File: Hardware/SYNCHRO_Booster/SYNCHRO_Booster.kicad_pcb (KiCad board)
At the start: 2 copper layers, 41 parts, among them IC1 L6203, J1 Conn_01x02_Pin, J2 Power_Input, J3 B4B-XH-A, SW1 SW_Push, SW2 SW_SPDT, U1 LM393P, U2 6N137, U3 6N137, U4 74LVC2G02

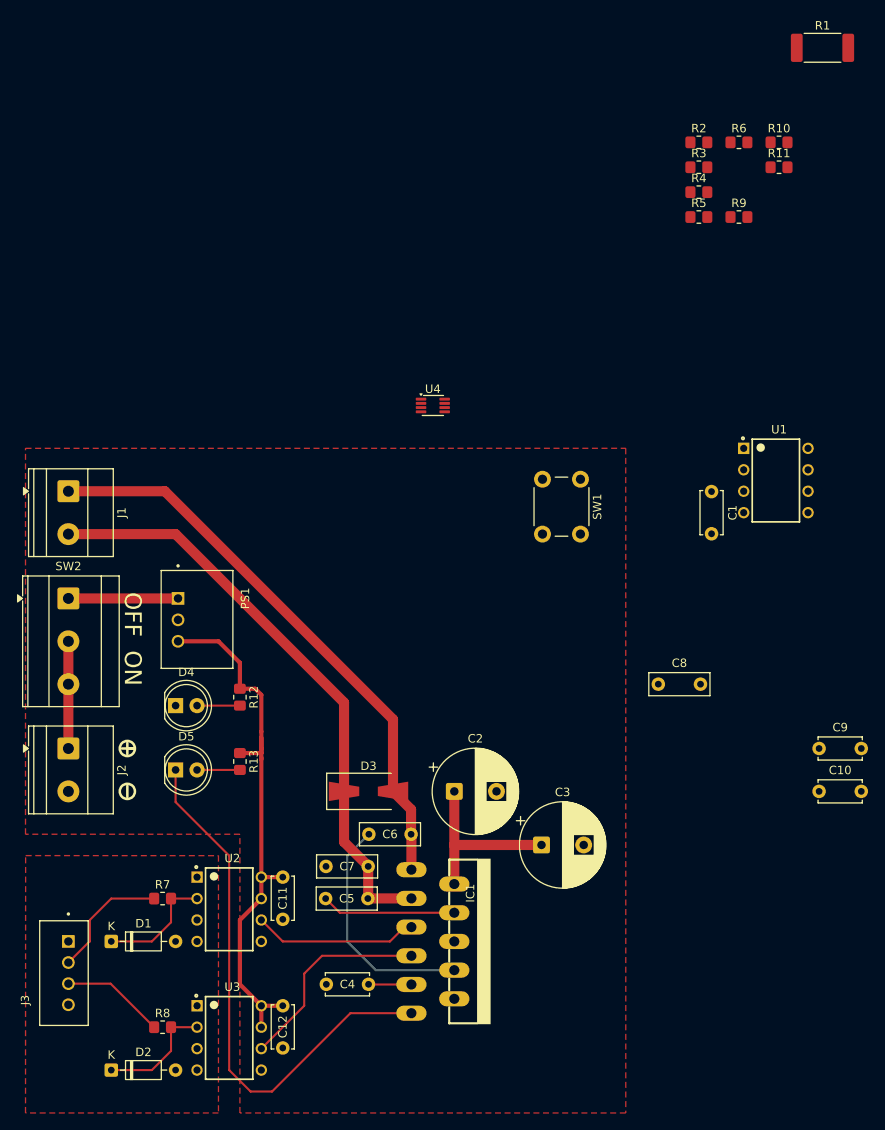
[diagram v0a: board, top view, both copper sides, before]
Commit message: Booster_Design_v1.0
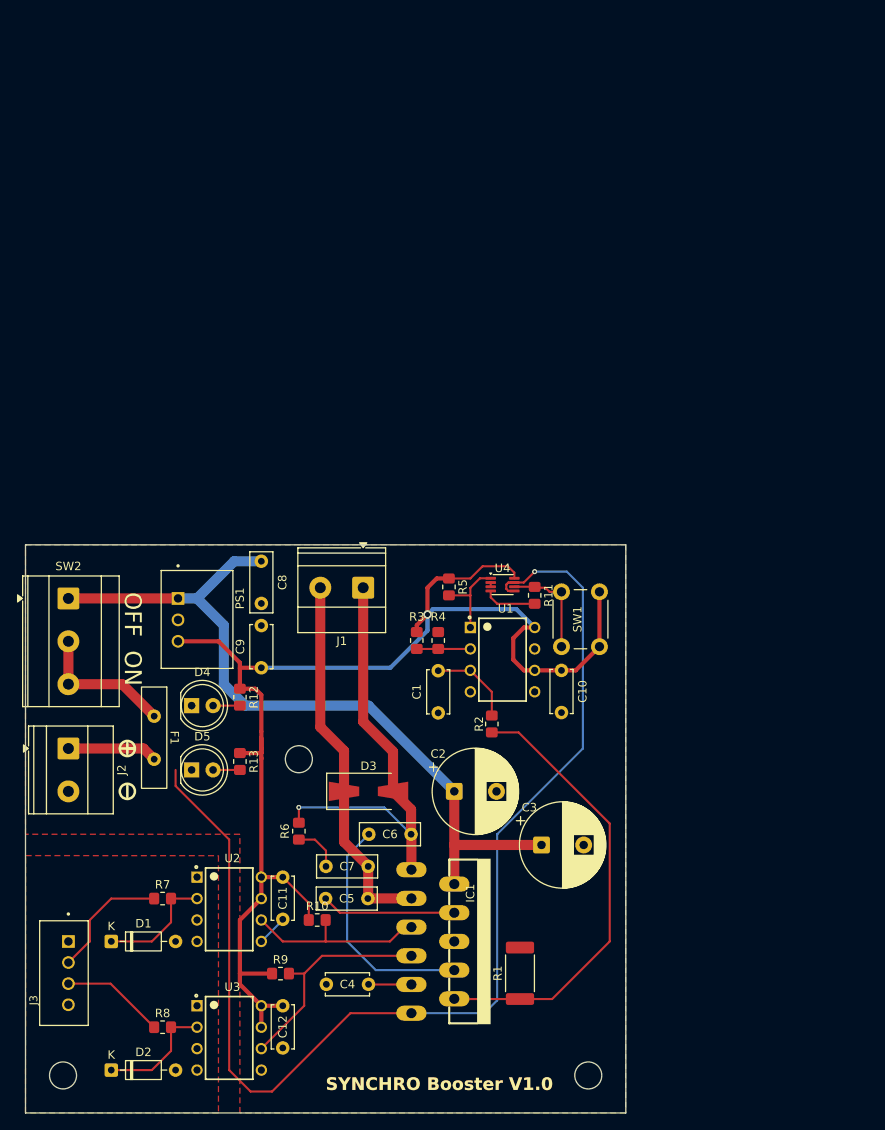
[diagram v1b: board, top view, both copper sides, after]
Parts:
- added F1: MF-R185-2-99, SYNCHRO_Library:Fuse_Bourns_MF-R185, F.Cu at (71.1, 110.5)
- added REF**: MountingHole_3.2mm_M3, MountingHole:MountingHole_3.2mm_M3, F.Cu at (60.3, 150.5)
- added REF**: MountingHole_3.2mm_M3, MountingHole:MountingHole_3.2mm_M3, F.Cu at (122.6, 150.5)
- added REF**: MountingHole_3.2mm_M3, MountingHole:MountingHole_3.2mm_M3, F.Cu at (88.3, 113.0)
- moved R1 115.4 mm to (114.5, 138.4), turned to 90 degrees
- moved R10 107.2 mm to (90.4, 132.1)
- moved R9 104.8 mm to (86.1, 138.4)
- moved R6 96.8 mm to (88.3, 121.6), turned to 90 degrees
- moved R2 73.1 mm to (111.1, 108.9), turned to -90 degrees
- moved C9 66.8 mm to (83.8, 102.2), turned to 90 degrees
- moved R3 65.3 mm to (102.2, 99.0), turned to -90 degrees
- moved R4 61.4 mm to (104.8, 99.0), turned to 90 degrees
- moved R11 58.4 mm to (116.2, 93.6), turned to -90 degrees
- moved R5 52.9 mm to (106.0, 92.6), turned to -90 degrees
- moved C8 49.2 mm to (83.8, 89.6), turned to -90 degrees
- moved U1 38.7 mm to (112.4, 101.2)
- moved C1 38.7 mm to (104.8, 102.5)
- moved J1 36.7 mm to (95.9, 92.7), turned to 180 degrees
- moved C10 33.7 mm to (119.4, 102.5), turned to -90 degrees
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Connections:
- SW2 pad 2: Net-(J2-Pin_1) -> Net-(SW2-B)
- SW2 pad 3: Net-(J2-Pin_1) -> Net-(SW2-B)
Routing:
- net +5V: track 65.4 -> 157.5 mm, vias 0 -> 1
- net /ENABLE: track 64.7 -> 140.6 mm, vias 0 -> 1
- net +15V: track 34.3 -> 90.0 mm
- net Net-(IC1-SENSE): track 0.00 -> 53.7 mm
- net Net-(D3-A1): track 70.5 -> 44.4 mm
- net Net-(SW2-B): track 0.00 -> 16.8 mm
- net Net-(D3-A2): track 68.4 -> 52.2 mm, vias 0 -> 1
- net Net-(R11-Pad1): track 0.00 -> 12.3 mm
- net /SENSE: track 0.00 -> 10.2 mm
- net Net-(U1-1OUT): track 0.00 -> 10.1 mm
- net GND1: track 0.00 -> 9.95 mm
- net Net-(U1-1IN-): track 0.00 -> 6.35 mm
- net Net-(C7-Pad2): track 0.00 -> 5.62 mm
- net /Booster_Signal_A: track 19.5 -> 22.1 mm
- net Net-(J2-Pin_1): track 12.7 -> 10.7 mm
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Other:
- board outline added: 71.1 x 67.3 mm
- board text added: "SYNCHRO Booster V1.0"

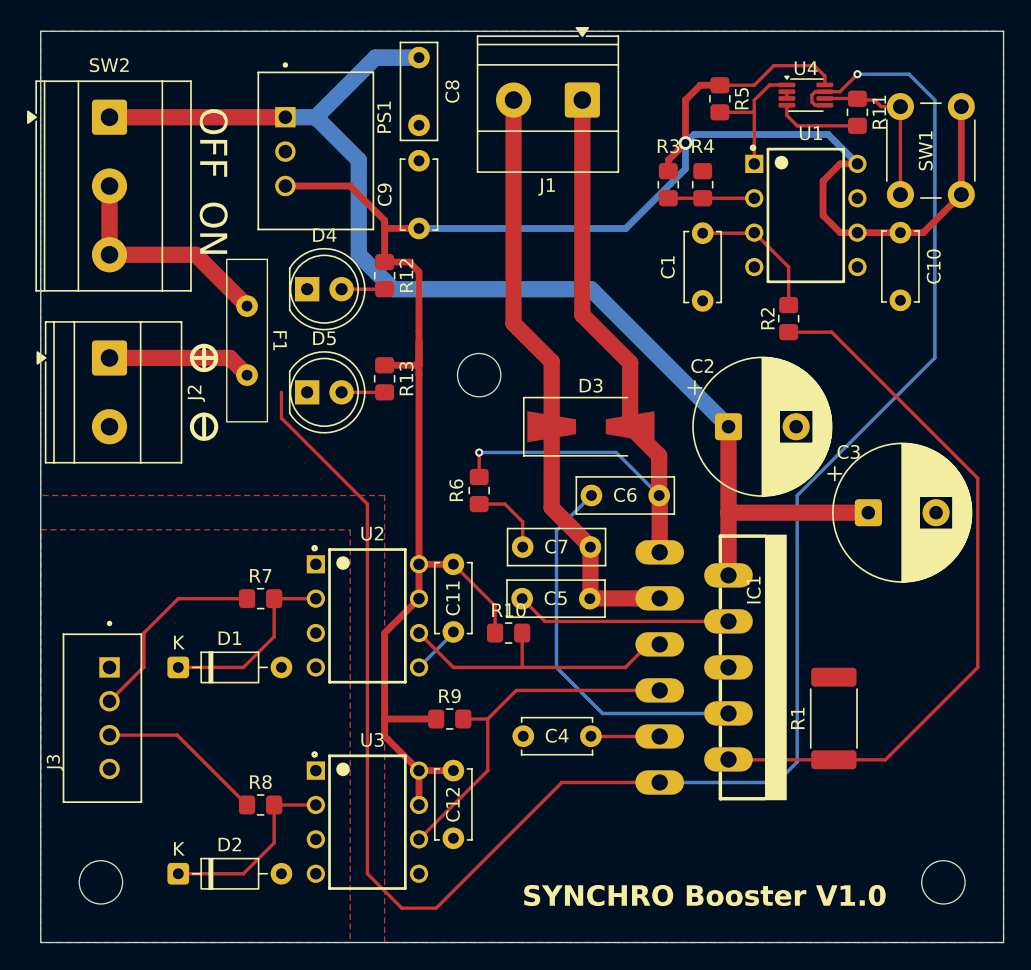
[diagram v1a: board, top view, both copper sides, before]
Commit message: hardware update push
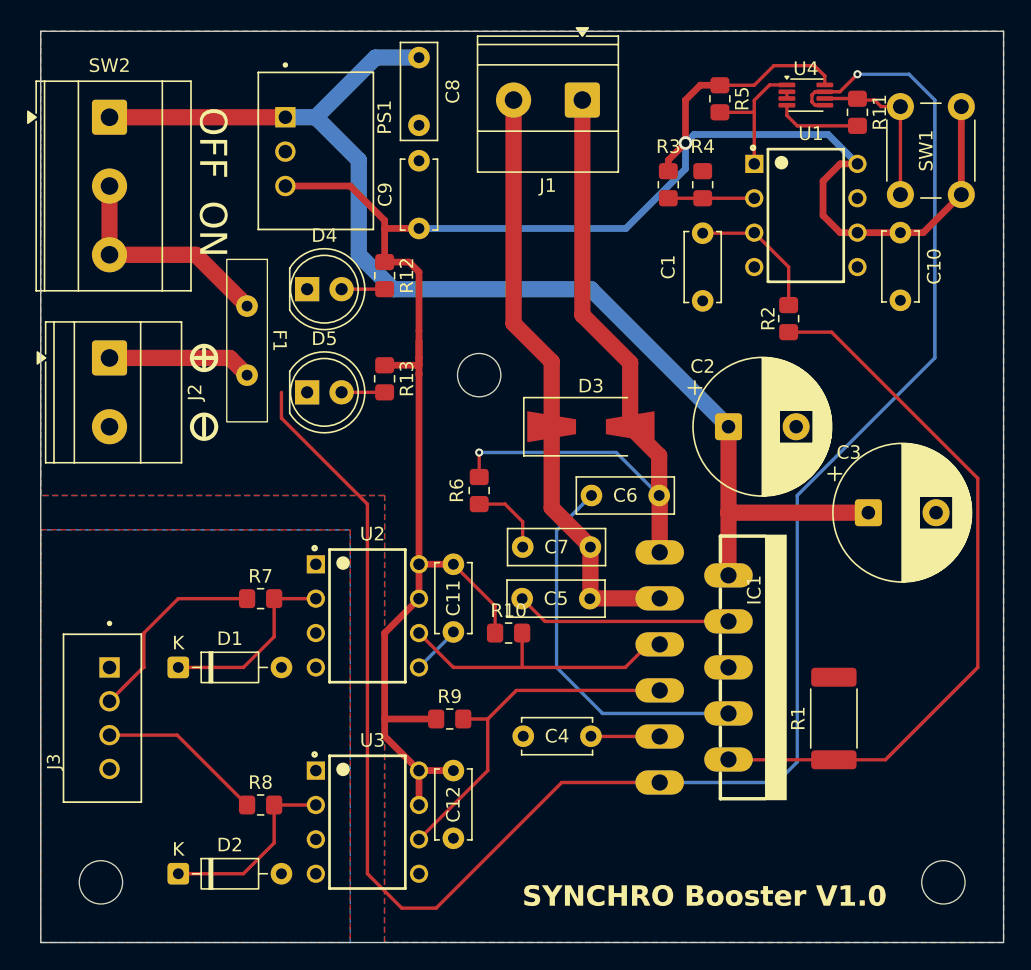
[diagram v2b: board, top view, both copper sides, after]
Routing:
- added copper zone on B.Cu, net GND1
- added copper zone on B.Cu, net GND_Z
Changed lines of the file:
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@@
 		(filling no)
 		(pcbplotparams
-			(layerselection 0x00000000_00000000_55555555_5755f5ff)
+			(layerselection 0x00000000_00000000_55555555_57555555)
 			(plot_on_all_layers_selection 0x00000000_00000000_00000000_00000000)
 			(disableapertmacros no)
@@
 			(outputformat 1)
 			(mirror no)
-			(drillshape 1)
+			(drillshape 0)
 			(scaleselection 1)
-			(outputdirectory "")
+			(outputdirectory "../GerberFiles/SYNCHRO_Booster_V1.0/")
 		)
 	)
@@
 	)
 	(segment
+		(start 71.12 107.93)
+		(end 67.33 104.14)
+		(width 1.2)
+		(layer "F.Cu")
+		(net "Net-(SW2-B)")
+	)
+	(segment
+		(start 67.33 104.14)
+		(end 60.96 104.14)
+		(width 1.2)
+		(layer "F.Cu")
+		(net "Net-(SW2-B)")
+	)
+	(segment
+		(start 60.96 104.14)
+		(end 60.96 99.06)
+		(width 1.2)
+		(layer "F.Cu")
+		(net "Net-(SW2-B)")
+	)
+	(segment
+		(start 60.96 111.76)
+		(end 69.85 111.76)
+		(width 1.2)
+		(layer "F.Cu")
+		(net "Net-(J2-Pin_1)")
+	)
+	(segment
+		(start 69.85 111.76)
+		(end 71.12 113.03)
+		(width 1.2)
+		(layer "F.Cu")
+		(net "Net-(J2-Pin_1)")
+	)
+	(segment
 		(start 63.46 134.62)
 		(end 63.5 134.62)
@@
 	)
 	(segment
-		(start 60.96 111.76)
-		(end 69.85 111.76)
-		(width 1.2)
-		(layer "F.Cu")
-		(net "Net-(J2-Pin_1)")
-	)
-	(segment
-		(start 69.85 111.76)
-		(end 71.12 113.03)
-		(width 1.2)
-		(layer "F.Cu")
-		(net "Net-(J2-Pin_1)")
-	)
-	(segment
 		(start 108.585 97.425)
 		(end 108.585 93.615)
@@
 		(net "Net-(U4-Pad2)")
 	)
-	(segment
-		(start 71.12 107.93)
-		(end 67.33 104.14)
-		(width 1.2)
-		(layer "F.Cu")
-		(net "Net-(SW2-B)")
-	)
-	(segment
-		(start 67.33 104.14)
-		(end 60.96 104.14)
-		(width 1.2)
-		(layer "F.Cu")
-		(net "Net-(SW2-B)")
-	)
-	(segment
-		(start 60.96 104.14)
-		(end 60.96 99.06)
-		(width 1.2)
-		(layer "F.Cu")
-		(net "Net-(SW2-B)")
-	)
 	(zone
 		(net "GND_Z")
@@
 			)
 		)
+	)
+	(zone
+		(net "GND_Z")
+		(layer "B.Cu")
+		(name "GND")
+		(hatch edge 0.5)
+		(priority 3)
+		(connect_pads
+			(clearance 0.5)
+		)
+		(min_thickness 0.25)
+		(fill yes
+			(thermal_gap 0.5)
+			(thermal_bridge_width 0.5)
+			(island_removal_mode 0)
+		)
+		(polygon
+			(pts
+				(xy 55.88 154.94) (xy 78.74 154.94) (xy 78.74 124.46) (xy 55.88 124.46)
+			)
+		)
+	)
+	(zone
+		(net "GND1")
+		(layer "B.Cu")
+		(name "GND")
+		(hatch edge 0.5)
+		(priority 2)
+		(connect_pads
+			(clearance 0.5)
+		)
+		(min_thickness 0.25)
+		(fill yes
+			(thermal_gap 0.5)
+			(thermal_bridge_width 0.5)
+			(island_removal_mode 0)
+		)
+		(polygon
+			(pts
+				(xy 55.88 87.63) (xy 127 87.63) (xy 127 154.94) (xy 81.268804 154.924487) (xy 81.28 121.92) (xy 55.88 121.92)
+			)
+		)
